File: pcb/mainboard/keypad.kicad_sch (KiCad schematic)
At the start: 20 parts, among them Y100 Crystal

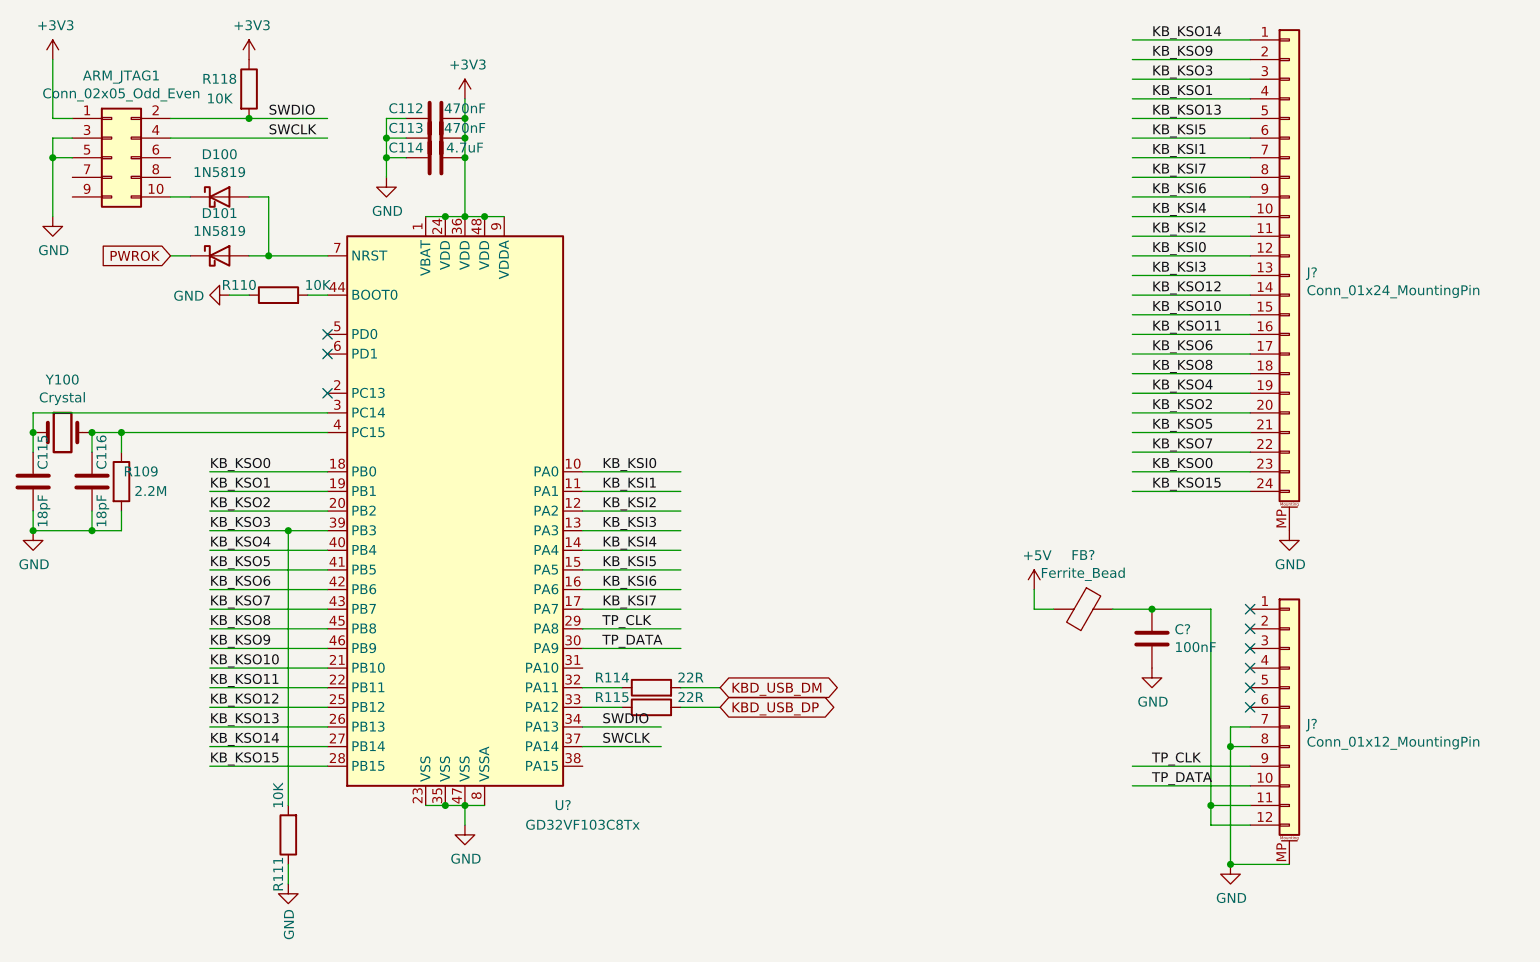
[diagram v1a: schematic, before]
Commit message: - pcb: working on r0p1 sch
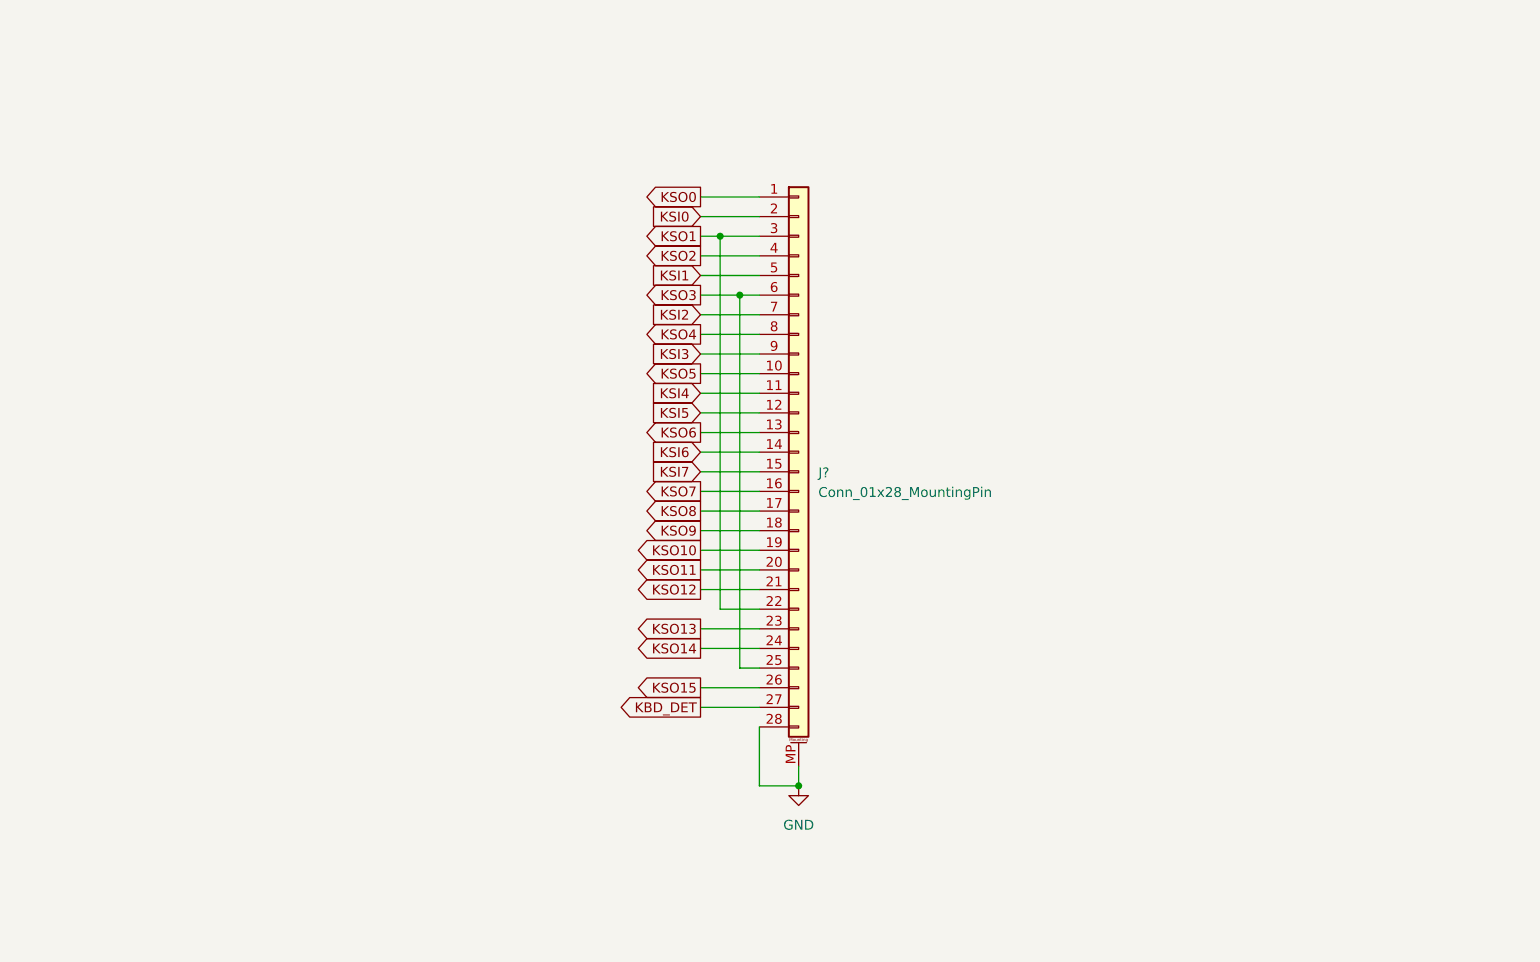
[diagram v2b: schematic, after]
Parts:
- removed ARM_JTAG1: Conn_02x05_Odd_Even, Connector_PinHeader_1.27mm:PinHeader_2x05_P1.27mm_Vertical_SMD, symbol Connector_Generic:Conn_02x05_Odd_Even
- removed C112, C113: 470nF, Capacitor_SMD:C_0402_1005Metric, symbol Device:C
- removed C114: 4.7uF, Capacitor_SMD:C_0603_1608Metric, symbol Device:C
- removed C115, C116: 18pF, Capacitor_SMD:C_0402_1005Metric, symbol Device:C
- removed C?: 100nF, symbol Device:C
- removed D100, D101: 1N5819, Diode_SMD:D_SOD-123, symbol Device:D_Schottky
- removed FB?: Ferrite_Bead, symbol Device:Ferrite_Bead
- removed J?: Conn_01x24_MountingPin, symbol Connector_Generic_MountingPin:Conn_01x24_MountingPin
- removed J?: Conn_01x12_MountingPin, symbol Connector_Generic_MountingPin:Conn_01x12_MountingPin
- removed R109: 2.2M, Capacitor_SMD:C_0402_1005Metric, symbol Device:R
- removed R110, R111, R118: 10K, Capacitor_SMD:C_0402_1005Metric, symbol Device:R
- removed R114, R115: 22R, Capacitor_SMD:C_0402_1005Metric, symbol Device:R
- removed U?: GD32VF103C8Tx, Package_QFP:LQFP-48_7x7mm_P0.5mm, symbol MCU_ST_STM32F1:STM32F103C8Tx
- removed Y100: Crystal, Crystal:Crystal_SMD_TXC_9HT11-2Pin_2.0x1.2mm_HandSoldering, symbol Device:Crystal
- added J?: Conn_01x28_MountingPin, symbol Connector_Generic_MountingPin:Conn_01x28_MountingPin
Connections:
- net GND: now also J?.28 (Pin_28), J?.MP (MountPin)
- new net KBD_DET: J?.27 (Pin_27)
- new net KSI0: J?.2 (Pin_2)
- new net KSI1: J?.5 (Pin_5)
- new net KSI2: J?.7 (Pin_7)
- new net KSI3: J?.9 (Pin_9)
- new net KSI4: J?.11 (Pin_11)
- new net KSI5: J?.12 (Pin_12)
- new net KSI6: J?.14 (Pin_14)
- new net KSI7: J?.15 (Pin_15)
- new net KSO0: J?.1 (Pin_1)
- new net KSO1: J?.22 (Pin_22), J?.3 (Pin_3)
- new net KSO10: J?.19 (Pin_19)
- new net KSO11: J?.20 (Pin_20)
- new net KSO12: J?.21 (Pin_21)
- new net KSO13: J?.23 (Pin_23)
- new net KSO14: J?.24 (Pin_24)
- new net KSO15: J?.26 (Pin_26)
- new net KSO2: J?.4 (Pin_4)
- new net KSO3: J?.25 (Pin_25), J?.6 (Pin_6)
- new net KSO4: J?.8 (Pin_8)
- new net KSO5: J?.10 (Pin_10)
- new net KSO6: J?.13 (Pin_13)
- new net KSO7: J?.16 (Pin_16)
- new net KSO8: J?.17 (Pin_17)
- new net KSO9: J?.18 (Pin_18)
- no-connect marks 9 -> 0
